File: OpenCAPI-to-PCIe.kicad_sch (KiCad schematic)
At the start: 9 parts, among them J1 OpenCAPI_AAC_Host, J2 Conn_01x06, J3 Bus_PCI_Express_x8

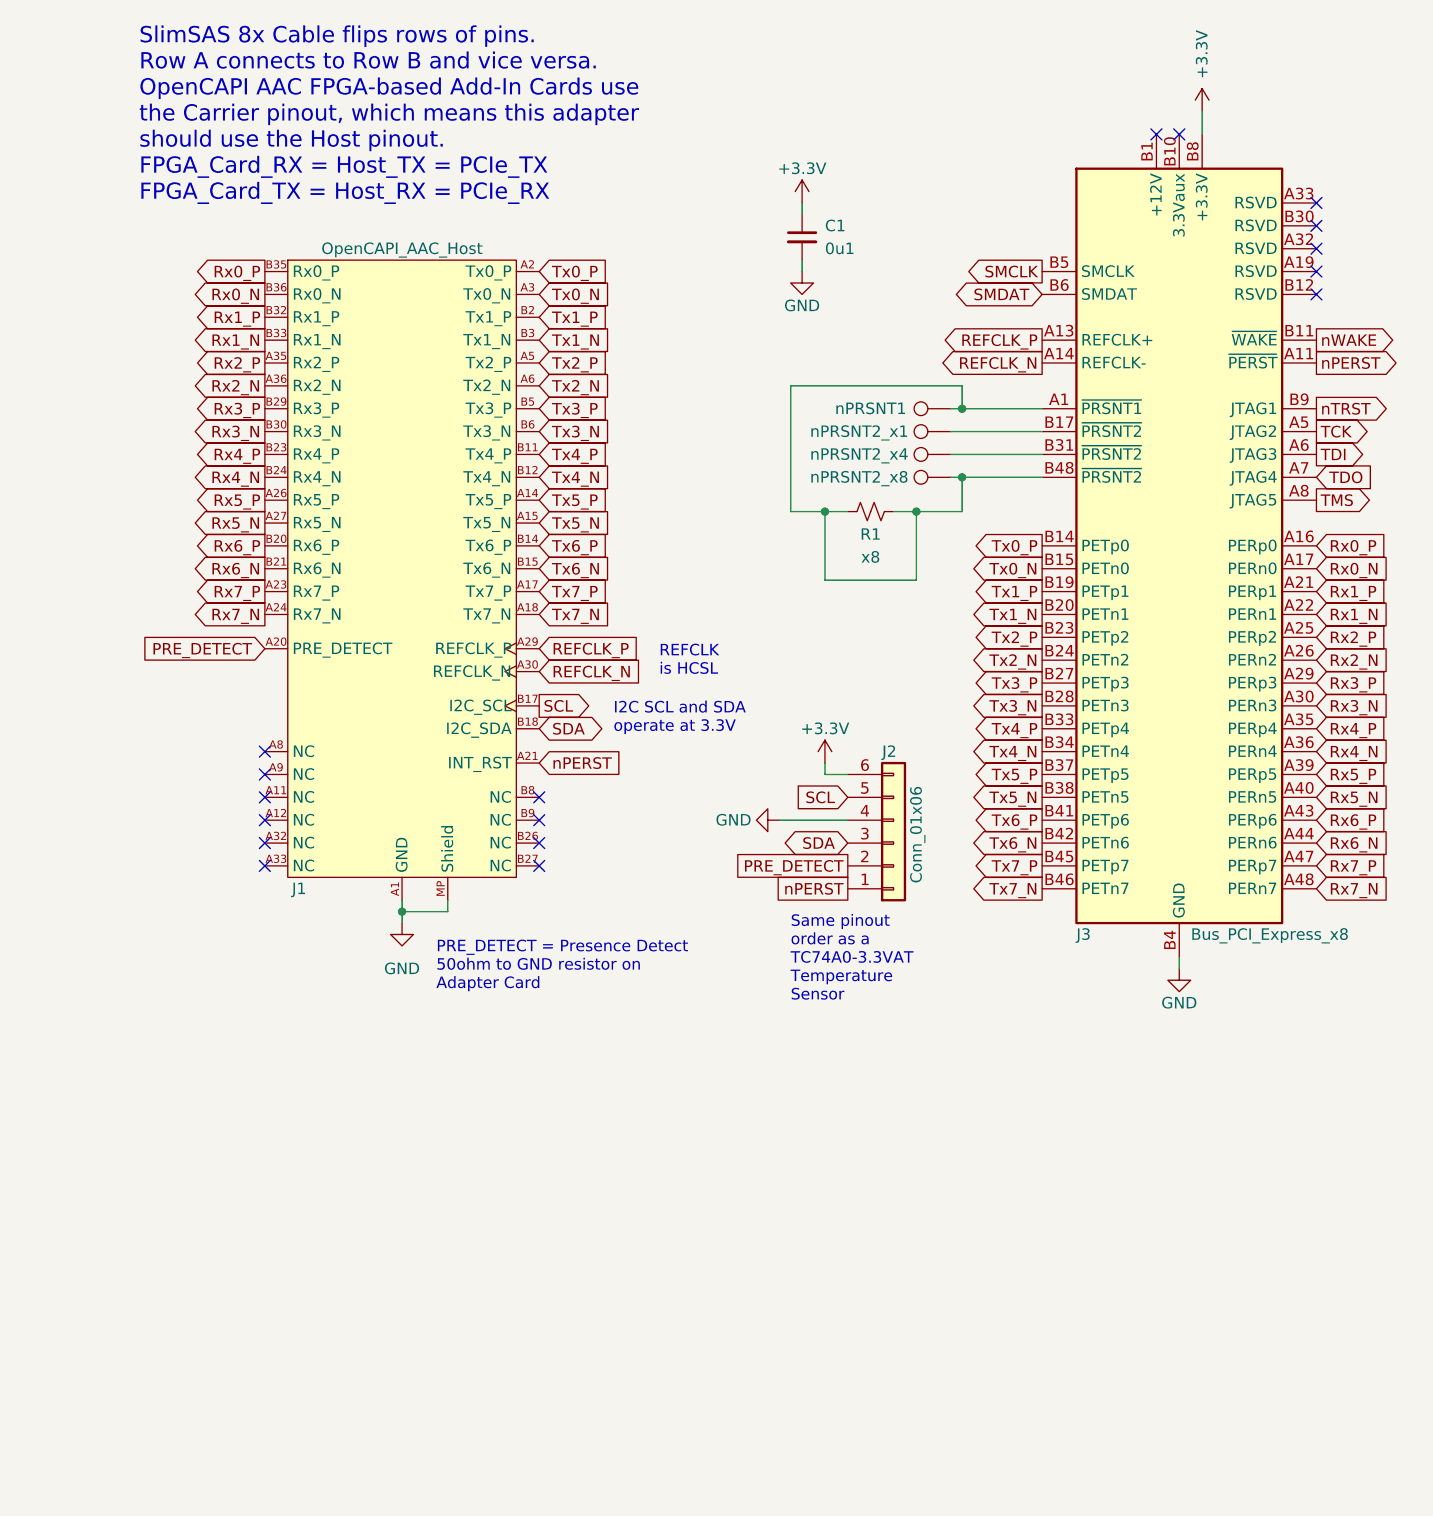
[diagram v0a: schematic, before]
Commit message: Third Revision
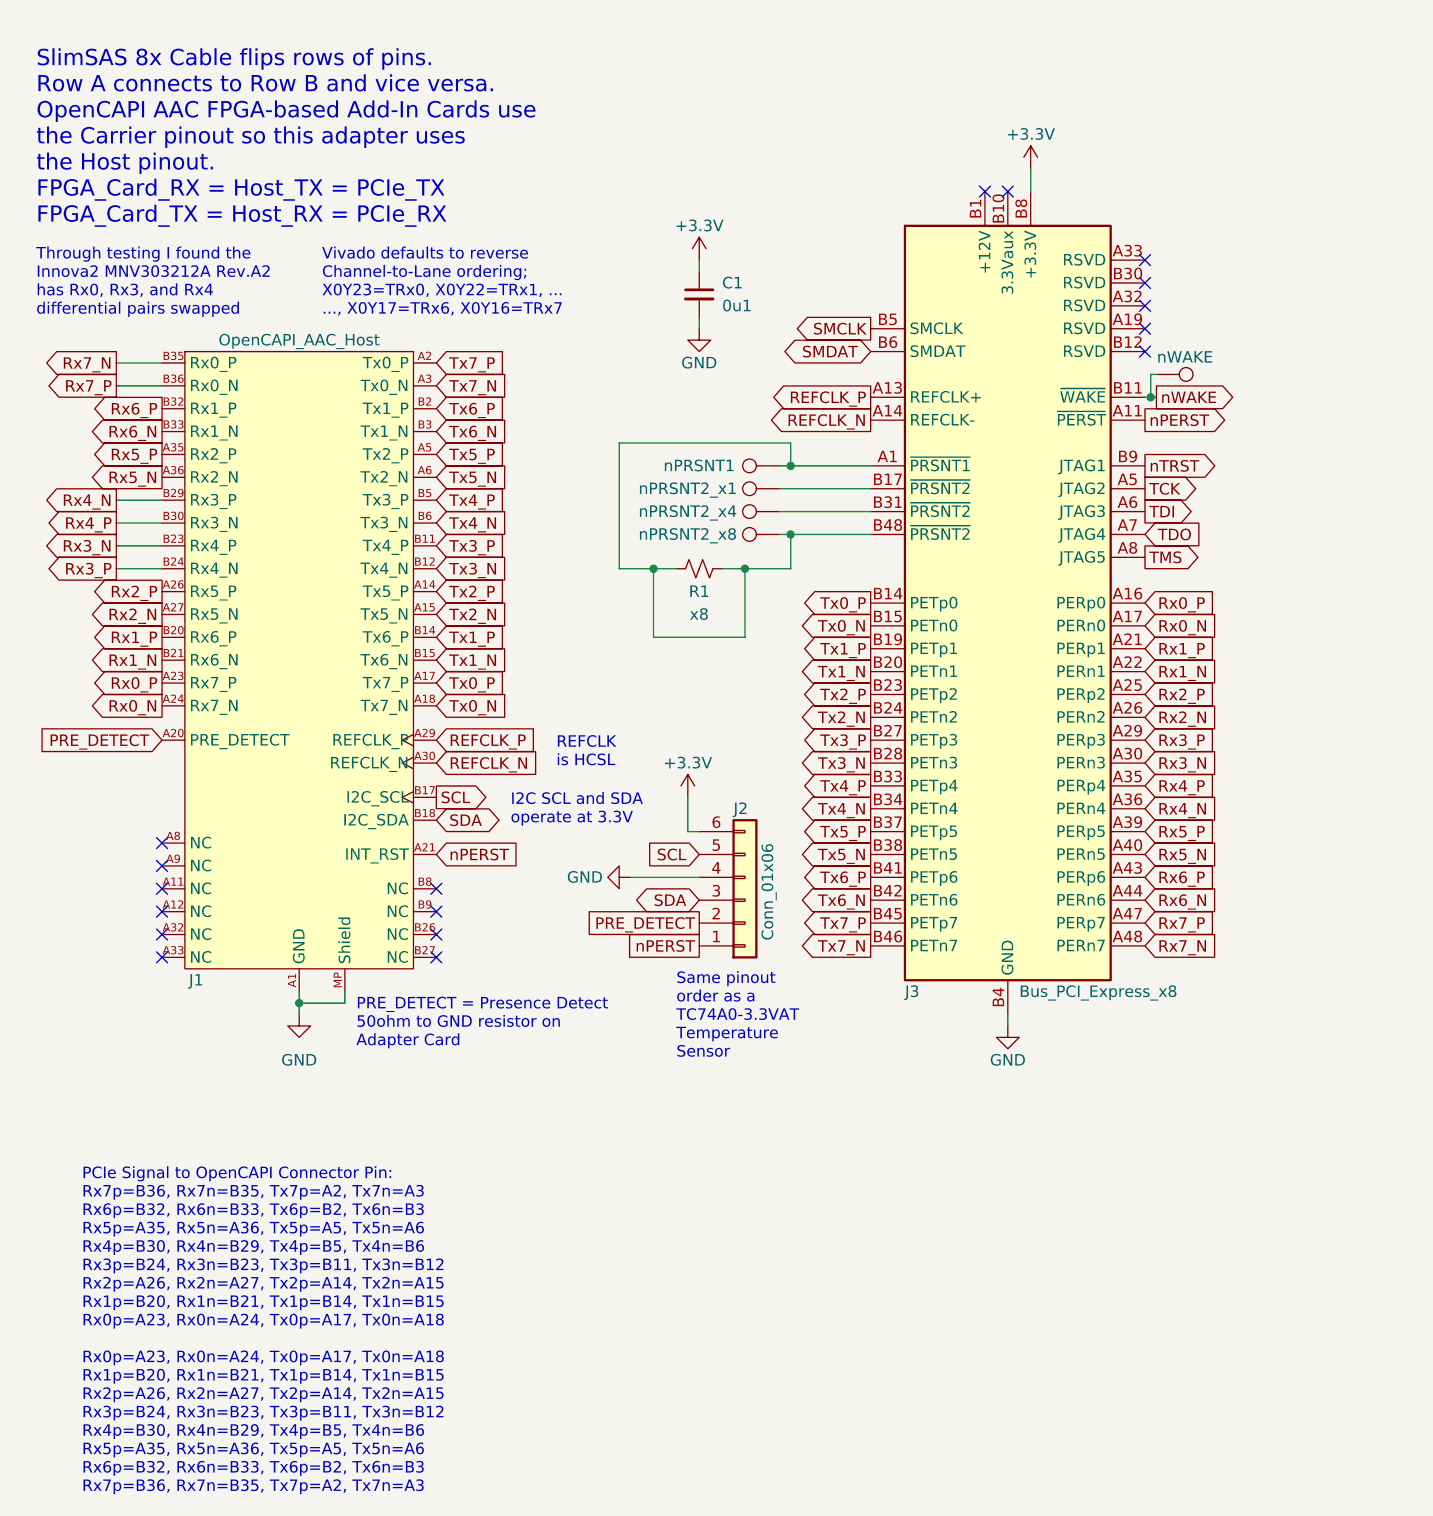
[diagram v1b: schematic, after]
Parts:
- added TP4: nWAKE, TestPoint:TestPoint_THTPad_D1.0mm_Drill0.5mm, symbol Connector:TestPoint
- C1: footprint Capacitor_SMD:C_0603_1608Metric_Pad1.08x0.95mm_HandSolder -> Capacitor_SMD:C_0805_2012Metric_Pad1.18x1.45mm_HandSolder
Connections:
- net Rx0_N: now also J1.A24 (Rx7_N); no longer J1.B36 (Rx0_N)
- net Rx0_P: now also J1.A23 (Rx7_P); no longer J1.B35 (Rx0_P)
- net Rx1_N: now also J1.B21 (Rx6_N); no longer J1.B33 (Rx1_N)
- net Rx1_P: now also J1.B20 (Rx6_P); no longer J1.B32 (Rx1_P)
- net Rx2_N: now also J1.A27 (Rx5_N); no longer J1.A36 (Rx2_N)
- net Rx2_P: now also J1.A26 (Rx5_P); no longer J1.A35 (Rx2_P)
- net Rx3_N: now also J1.B23 (Rx4_P); no longer J1.B30 (Rx3_N)
- net Rx3_P: now also J1.B24 (Rx4_N); no longer J1.B29 (Rx3_P)
- net Rx4_N: now also J1.B29 (Rx3_P); no longer J1.B24 (Rx4_N)
- net Rx4_P: now also J1.B30 (Rx3_N); no longer J1.B23 (Rx4_P)
- net Rx5_N: now also J1.A36 (Rx2_N); no longer J1.A27 (Rx5_N)
- net Rx5_P: now also J1.A35 (Rx2_P); no longer J1.A26 (Rx5_P)
- net Rx6_N: now also J1.B33 (Rx1_N); no longer J1.B21 (Rx6_N)
- net Rx6_P: now also J1.B32 (Rx1_P); no longer J1.B20 (Rx6_P)
- net Rx7_N: now also J1.B35 (Rx0_P); no longer J1.A24 (Rx7_N)
- net Rx7_P: now also J1.B36 (Rx0_N); no longer J1.A23 (Rx7_P)
- net Tx0_N: now also J1.A18 (Tx7_N); no longer J1.A3 (Tx0_N)
- net Tx0_P: now also J1.A17 (Tx7_P); no longer J1.A2 (Tx0_P)
- net Tx1_N: now also J1.B15 (Tx6_N); no longer J1.B3 (Tx1_N)
- net Tx1_P: now also J1.B14 (Tx6_P); no longer J1.B2 (Tx1_P)
- net Tx2_N: now also J1.A15 (Tx5_N); no longer J1.A6 (Tx2_N)
- net Tx2_P: now also J1.A14 (Tx5_P); no longer J1.A5 (Tx2_P)
- net Tx3_N: now also J1.B12 (Tx4_N); no longer J1.B6 (Tx3_N)
- net Tx3_P: now also J1.B11 (Tx4_P); no longer J1.B5 (Tx3_P)
- net Tx4_N: now also J1.B6 (Tx3_N); no longer J1.B12 (Tx4_N)
- net Tx4_P: now also J1.B5 (Tx3_P); no longer J1.B11 (Tx4_P)
- net Tx5_N: now also J1.A6 (Tx2_N); no longer J1.A15 (Tx5_N)
- net Tx5_P: now also J1.A5 (Tx2_P); no longer J1.A14 (Tx5_P)
- net Tx6_N: now also J1.B3 (Tx1_N); no longer J1.B15 (Tx6_N)
- net Tx6_P: now also J1.B2 (Tx1_P); no longer J1.B14 (Tx6_P)
- net Tx7_N: now also J1.A3 (Tx0_N); no longer J1.A18 (Tx7_N)
- net Tx7_P: now also J1.A2 (Tx0_P); no longer J1.A17 (Tx7_P)
- net nWAKE: now also TP4.1
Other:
- note added: "PCIe Signal to OpenCAPI Connector Pin: Rx7p=B36, Rx7n=B35, Tx7p=A2, Tx7n=A3 Rx6p=B32, Rx6n=B33, Tx6p=B2, Tx6n=B3 Rx5p=A35, Rx5n=A36, Tx5p=A5, Tx5n=A6 Rx4p=B30, Rx4n=B29, Tx4p=B5, Tx4n=B6 Rx3p=B24, Rx3n=B23, Tx3p=B11, Tx3n=B12 Rx2p=A26, Rx2n=A27, Tx2p=A14, Tx2n=A15 Rx1p=B20, Rx1n=B21, Tx1p=B14, Tx1n=B15 Rx0p=A23, Rx0n=A24, Tx0p=A17, Tx0n=A18 Rx0p=A23, Rx0n=A24, Tx0p=A17, Tx0n=A18 Rx1p=B20, Rx1n=B2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"
- note added: "SlimSAS 8x Cable flips rows of pins. Row A connects to Row B and vice versa. OpenCAPI AAC FPGA-based Add-In Cards use the Carrier pinout so this adapter uses the Host pinout. FPGA_Card_RX = Host_TX = PCIe_TX FPGA_Card_TX = Host_RX = PCIe_RX"
- note added: "Through testing I found the Innova2 MNV303212A Rev.A2 has Rx0, Rx3, and Rx4 differential pairs swapped"
- note added: "Vivado defaults to reverse Channel-to-Lane ordering; X0Y23=TRx0, X0Y22=TRx1, ... ..., X0Y17=TRx6, X0Y16=TRx7"
- note removed: "SlimSAS 8x Cable flips rows of pins. Row A connects to Row B and vice versa. OpenCAPI AAC FPGA-based Add-In Cards use the Carrier pinout, which means this adapter should use the Host pinout. FPGA_Card_RX = Host_TX = PCIe_TX FPGA_Card_TX = Host_RX = PCIe_RX"
- moved on the sheet: C1, J1, J2, J3, R1
